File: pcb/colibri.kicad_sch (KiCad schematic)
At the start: 55 parts

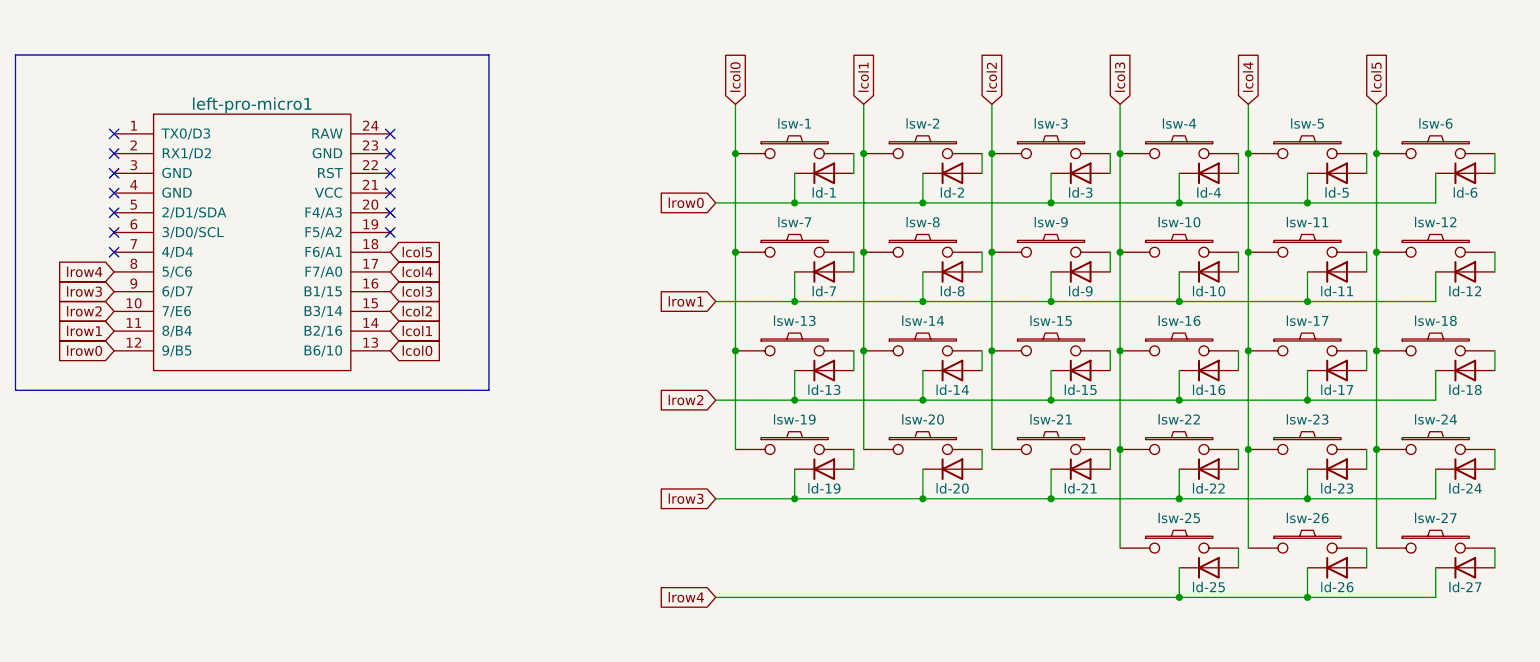
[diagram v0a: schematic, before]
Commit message: basic layout
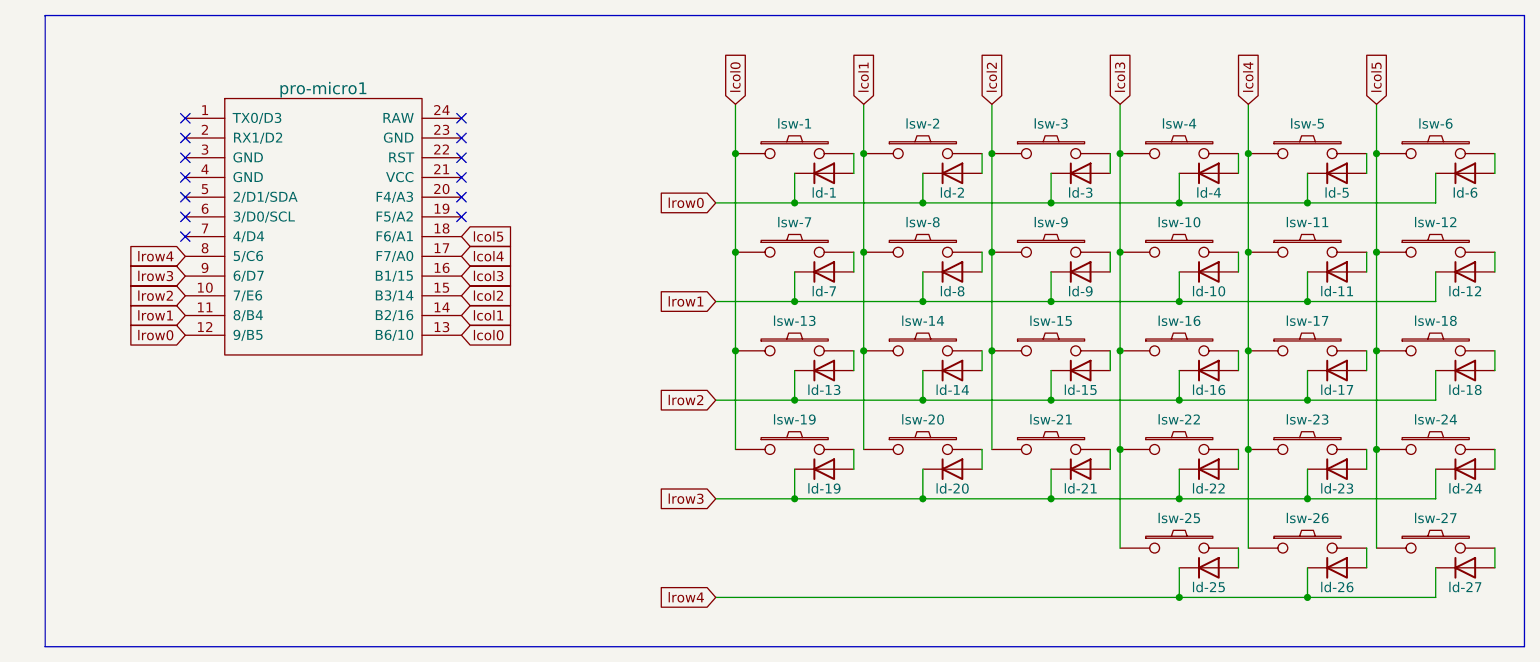
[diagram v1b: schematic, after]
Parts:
- ld-1, ld-10, ld-11, ld-12, ld-13, ld-14, ld-15, ld-16, ld-17, ld-18, ld-19, ld-2, ld-20, ld-21, ld-22, ld-23, ld-24, ld-25, ld-26, ld-27, ld-3, ld-4, ld-5, ld-6, ld-7, ld-8, ld-9: footprint kbd:D3_SMD_v2 -> kbd:D3_TH_SMD_v2
- lsw-1, lsw-13, lsw-19, lsw-7: footprint kbd:CherryMX_Hotswap_1.5u -> kbd:CherryMX_Hotswap_1.25U
- pro-micro1: renamed from left-pro-micro1; footprint kbd:ProMicro_v3.5 -> kbd:ProMicro_v4
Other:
- moved on the sheet: pro-micro1
